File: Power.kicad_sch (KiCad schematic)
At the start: 36 parts, among them IC1 LMR33640DDDAR, J13 SM02B-GHS-TB, J16 SM02B-GHS-TB, J17 Screw_Terminal_01x02, Q1 SI2369BDS-T1-GE3 30V 5.6A, U3 AP7361C-33ER-13

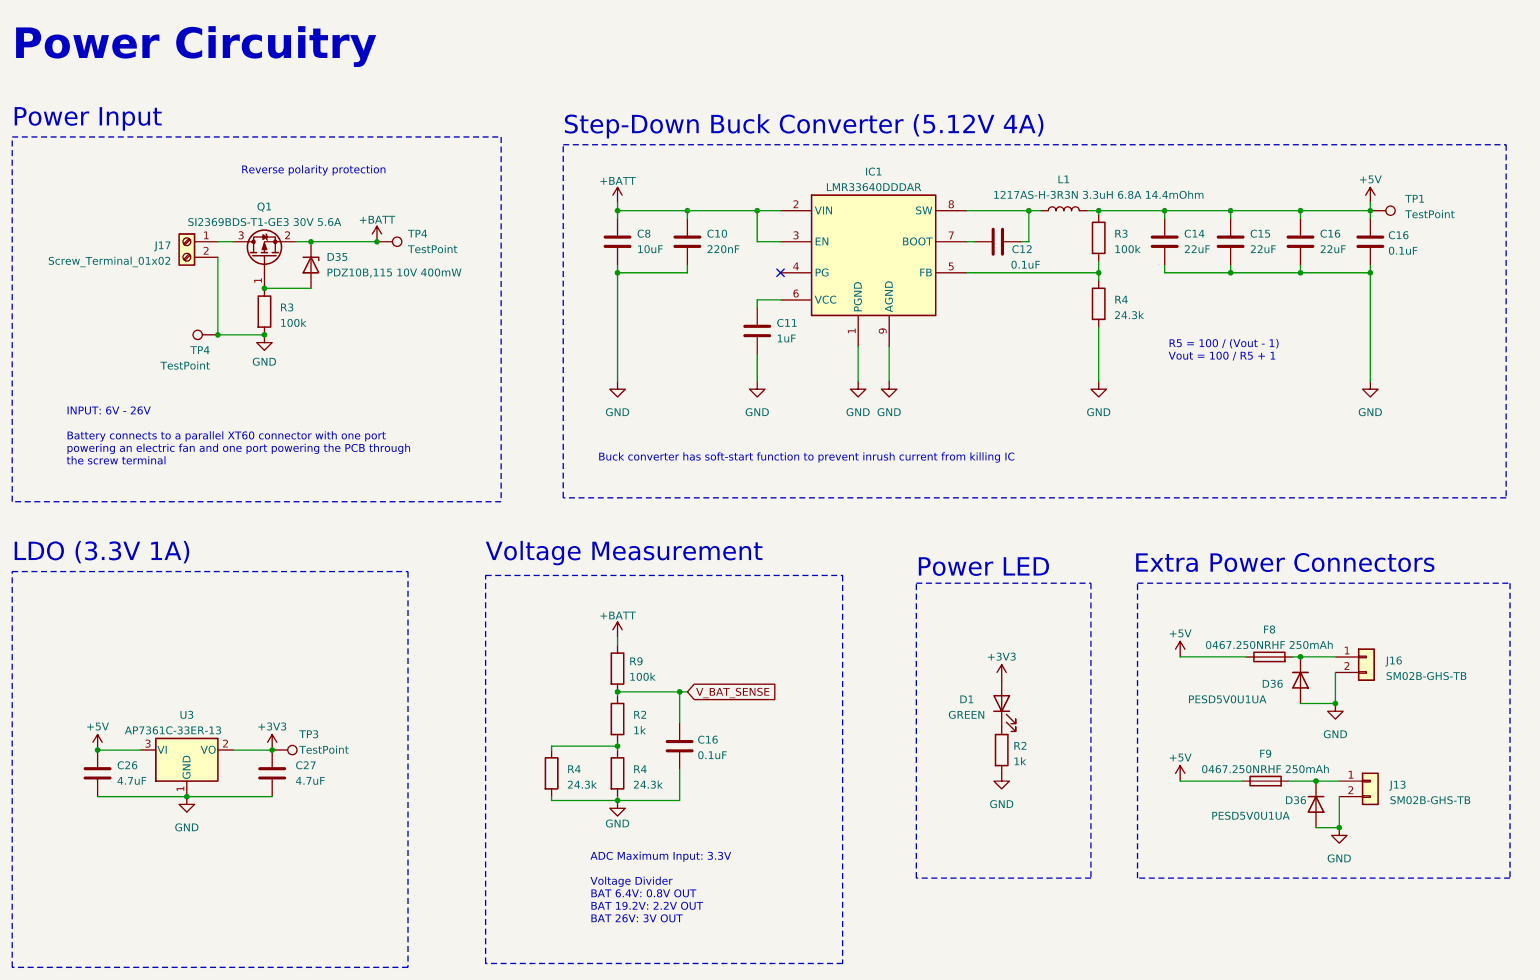
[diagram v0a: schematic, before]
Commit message: Add files via upload
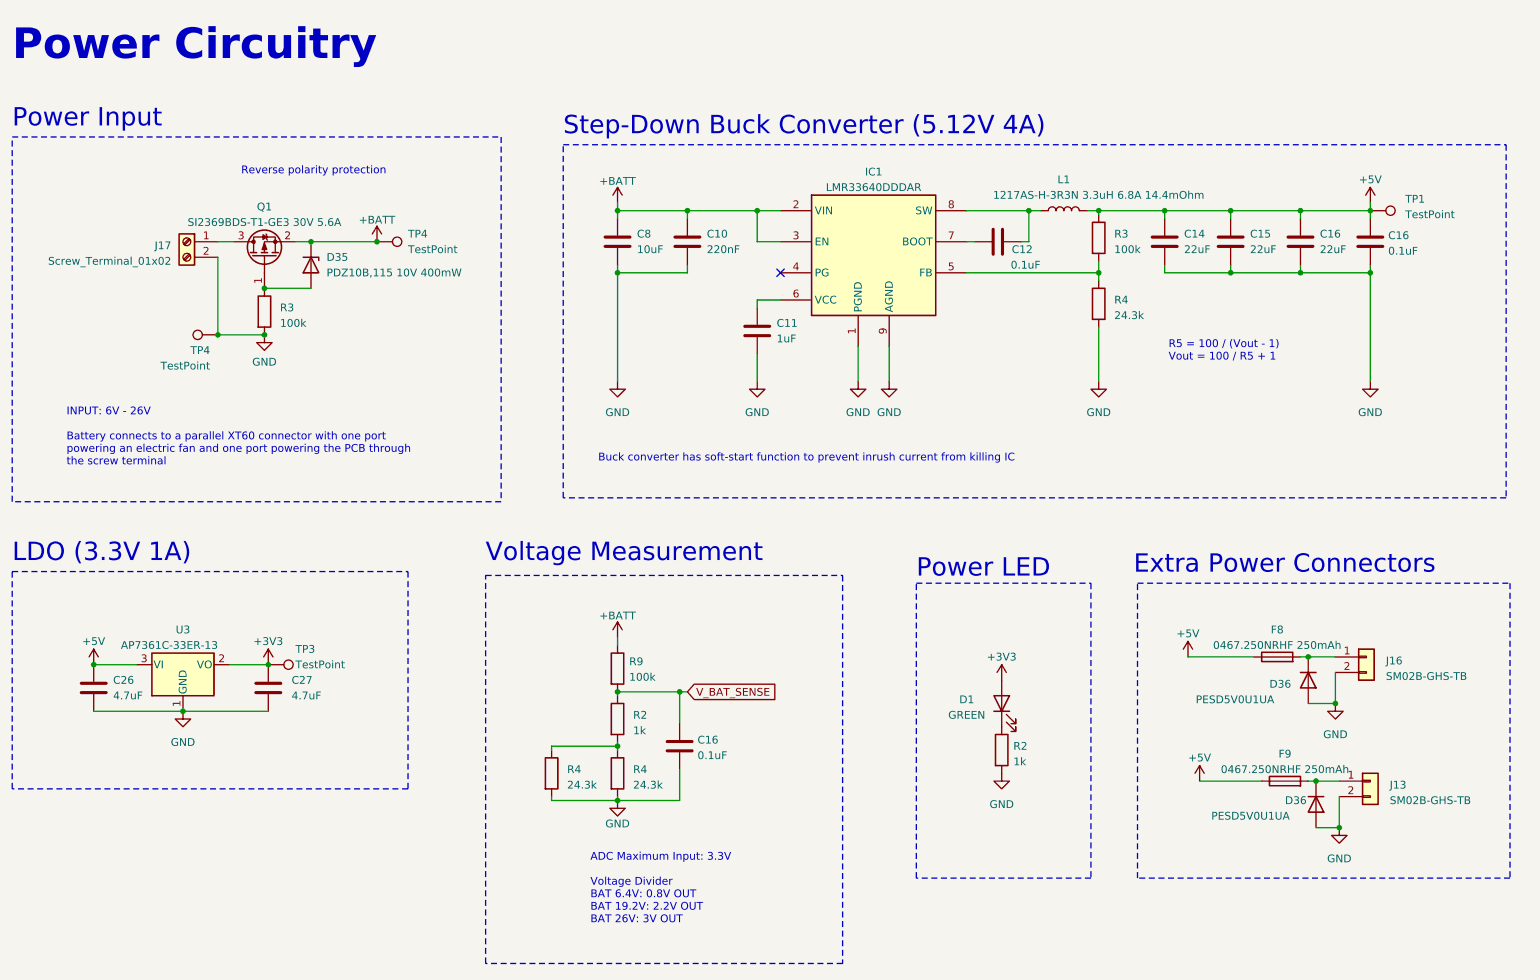
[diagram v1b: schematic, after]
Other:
- moved on the sheet: C26, C27, D36, F8, F9, TP3, U3
